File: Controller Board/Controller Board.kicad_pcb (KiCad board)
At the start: 2 copper layers, 50.8 x 26 mm, 18 parts, among them J1 Fan_connector, J2 Conn_01x04, J3 Conn_01x03, K1 G3MB-202PDC5 Relay, SW1 SW_SPDT, U1 attiny85, U2 AMS1117-5.0

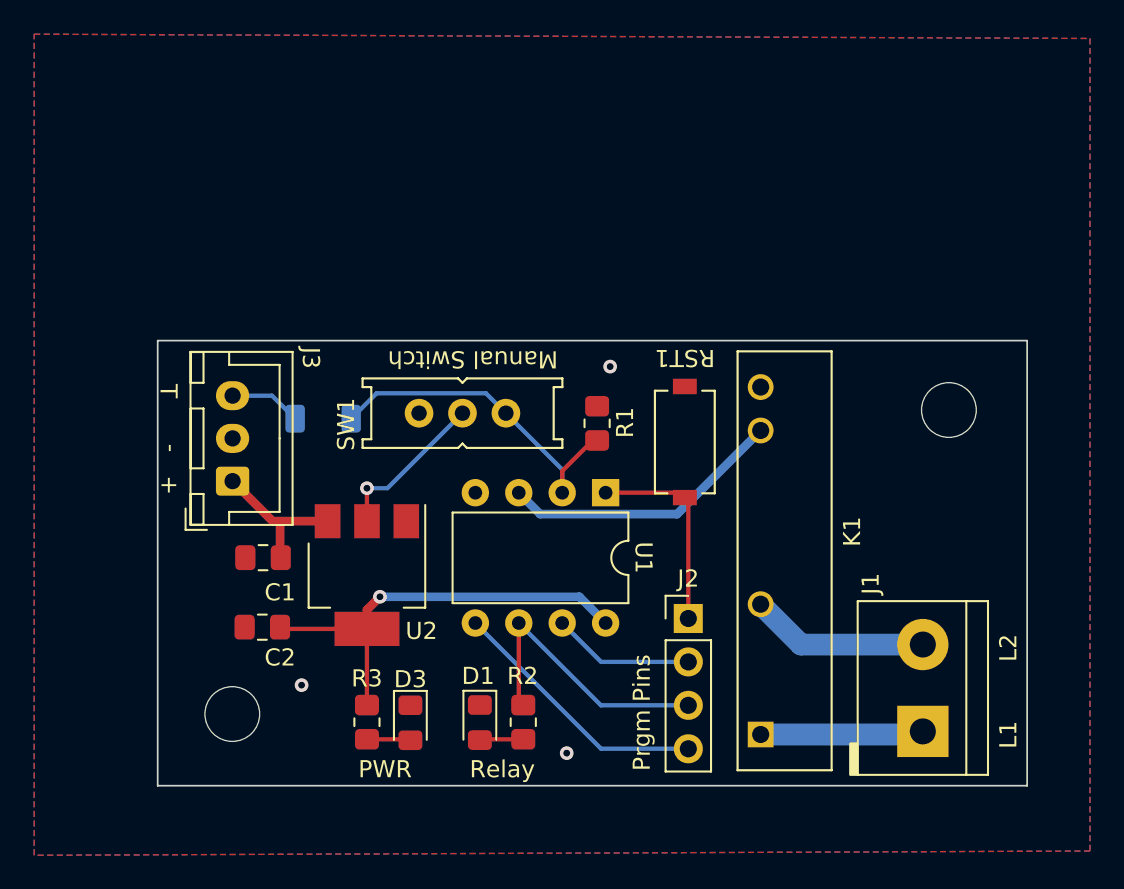
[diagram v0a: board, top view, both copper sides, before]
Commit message: created final Schematic and PCB
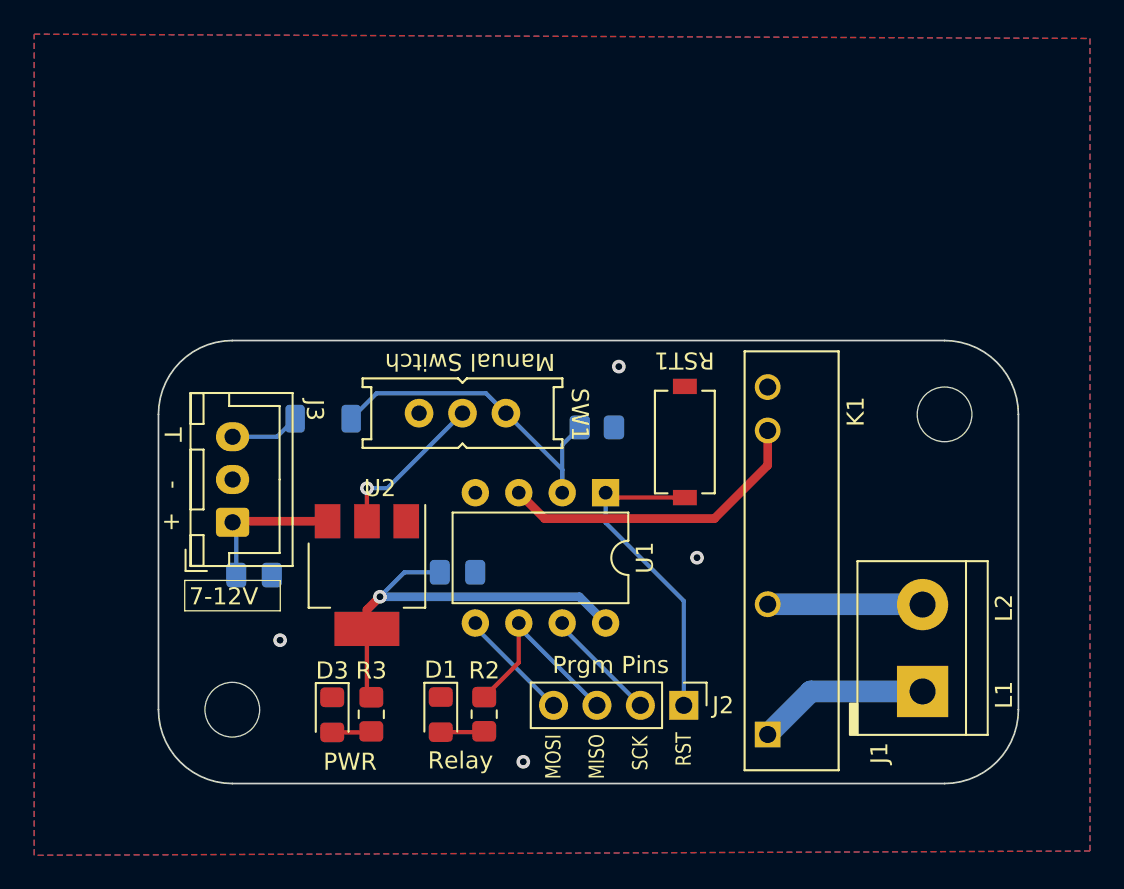
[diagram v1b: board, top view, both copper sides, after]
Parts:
- C1, C2, R1: moved to B.Cu
- moved C2 11.9 mm to (124.2, 91.3), turned to 180 degrees
- moved J2 5.09 mm to (137.4, 99.1), turned to -90 degrees
- moved D3 4.60 mm to (116.8, 99.6)
- moved J3 2.40 mm to (111.0, 88.4)
- moved J1 2.34 mm to (150.4, 96.0)
- moved D1 2.33 mm to (123.2, 99.6)
- moved R2 2.33 mm to (125.7, 99.6)
- moved C1 1.15 mm to (112.3, 91.4), turned to 180 degrees
- moved R3 0.53 mm to (119.1, 99.6)
- moved K1 0.41 mm to (145.4, 90.9)
- moved H1 0.36 mm to (152.7, 82.0)
- moved H2 0.25 mm to (111.0, 99.3)
- moved R1 0.24 mm to (132.3, 82.8), turned to 180 degrees
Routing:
- net /MOSI: track 15.5 -> 6.71 mm
- net /Reset: track 11.9 -> 19.1 mm
- net /MISO: track 16.8 -> 11.9 mm
- net Net-(K1-Signal+): track 16.7 -> 18.5 mm
- net /SCK: track 8.32 -> 6.71 mm
- net Net-(J1-Pin_2): track 10.5 -> 9.07 mm
- net /Vcc: track 34.9 -> 33.6 mm
- net Net-(J1-Pin_1): track 9.56 -> 10.1 mm
- net GND: vias 3 -> 4
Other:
- board size 50.8 x 26 mm -> 50.3 x 25.9 mm
- board text added: "7-12V"
- board text added: "Attiny85 Relay Controller"
- board text added: "Trigger -> PB3 Relay -> PB4 LED -> PB0"
- board text added: "When programming manual Swt must be off."
- board text removed: "Attiny85 Glowforge External Fan Controller"
